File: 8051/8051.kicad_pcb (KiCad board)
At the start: 2 copper layers, 70 x 90 mm, 49 parts, among them J1 GND, J10 C_{OUT}, J2 V_{CC}, J3 OUT TX RX V5 G, J4 S + G, J5 G + CK D, J6 AP-B-C, J7 AN-B-C, J8 A_{OUT}, J9 B_{OUT}, Q1 2N3055, Q2 nfet, Q3 pfet, Q4 2N3055, Q5 nfet, Q6 pfet, Q7 2N3055, Q8 nfet, Q9 pfet, U1 L7805, U2 REGULAR-7133-1, U3 C8051F330

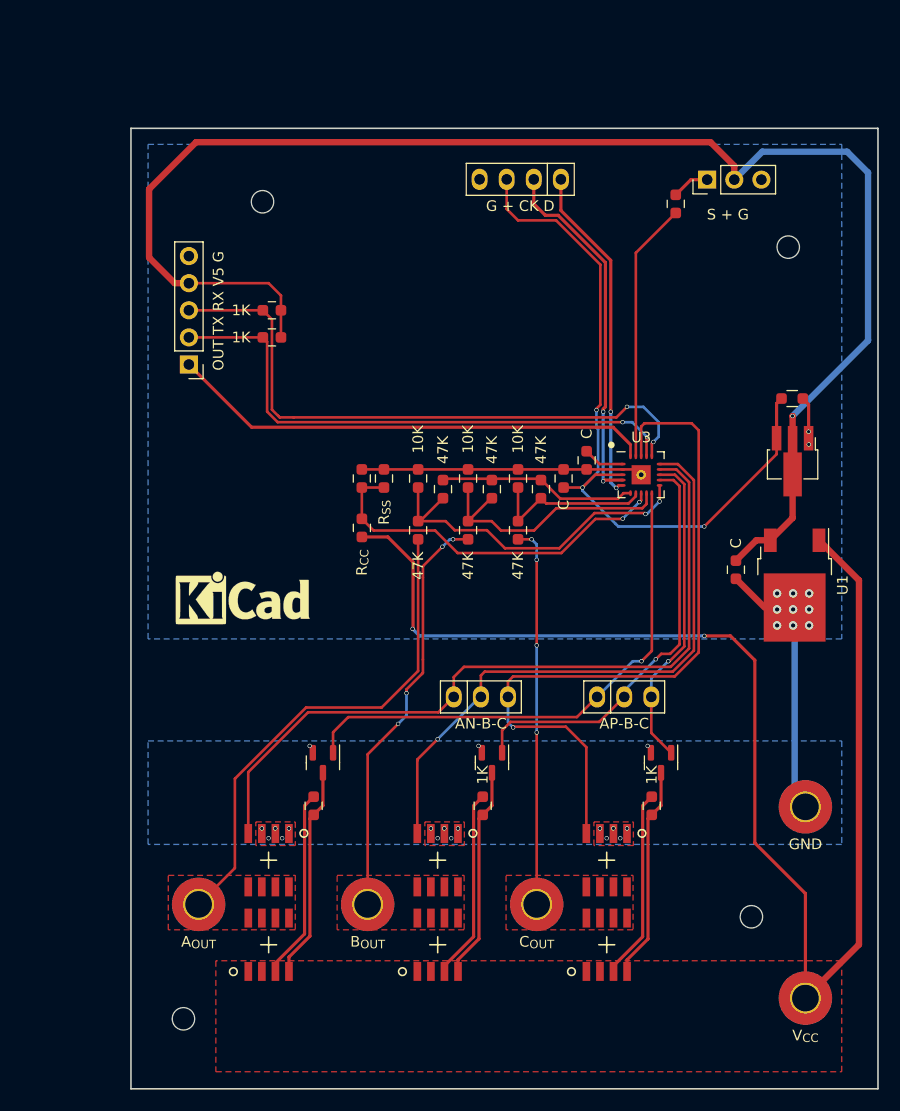
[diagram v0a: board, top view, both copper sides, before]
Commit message: digital module
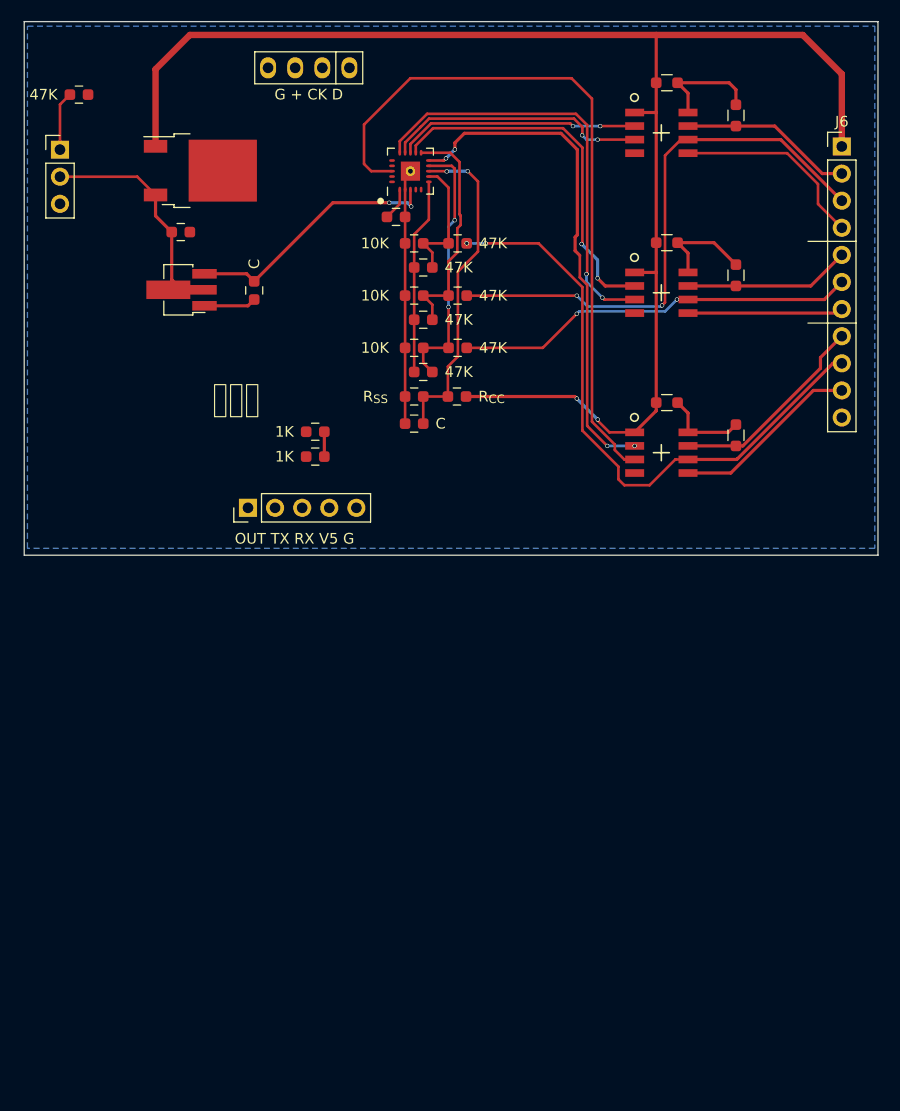
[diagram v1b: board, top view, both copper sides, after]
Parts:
- removed C: 0805_p2.0xpad1.0, footprint:0805_p2.0xpad1.0
- removed J1: GND, MountingHole:MountingHole_2.5mm_Pad_TopBottom
- removed J10: C_{OUT}, MountingHole:MountingHole_2.5mm_Pad_TopBottom
- removed J2: V_{CC}, MountingHole:MountingHole_2.5mm_Pad_TopBottom
- removed J7: AN-B-C, footprint:CONN3-P2.54-DR1.0-W1.5
- removed J8: A_{OUT}, MountingHole:MountingHole_2.5mm_Pad_TopBottom
- removed J9: B_{OUT}, MountingHole:MountingHole_2.5mm_Pad_TopBottom
- removed Q1, Q4, Q7: 2N3055, Package_TO_SOT_SMD:SOT-23
- removed Q2, Q5, Q8: nfet, footprint:SOIC-8
- removed Q3, Q6, Q9: pfet, footprint:SOIC-8
- removed R15, R16, R17: 1K, footprint:0603_p1.7xpad1.0
- removed REF** (x4): MountingHole_2.1mm, MountingHole:MountingHole_2.1mm
- removed REF**: KiCad-Logo_5mm_SilkScreen, Symbol:KiCad-Logo_5mm_SilkScreen
- added C5: C, footprint:0805_p2.0xpad1.0, F.Cu at (86.7, 28.8)
- added C6: C, footprint:0805_p2.0xpad1.0, F.Cu at (86.7, 43.8)
- added C7: C, footprint:0805_p2.0xpad1.0, F.Cu at (86.7, 58.8)
- added D1: D, footprint:0805_p2.0xpad1.0, F.Cu at (80.2, 25.7)
- added D2: D, footprint:0805_p2.0xpad1.0, F.Cu at (80.2, 40.7)
- added D3: D, footprint:0805_p2.0xpad1.0, F.Cu at (80.2, 55.7)
- added U4: IR2103, footprint:SOIC-8, F.Cu at (79.7, 30.4)
- added U5: IR2103, footprint:SOIC-8, F.Cu at (79.7, 45.4)
- added U6: IR2103, footprint:SOIC-8, F.Cu at (79.7, 60.4)
- J3: value OUT TX RX V5 G -> S + G; footprint Connector_PinHeader_2.54mm:PinHeader_1x05_P2.54mm_Vertical -> Connector_PinHeader_2.54mm:PinHeader_1x03_P2.54mm_Vertical
- J4: value S + G -> OUT TX RX V5 G; footprint Connector_PinHeader_2.54mm:PinHeader_1x03_P2.54mm_Vertical -> Connector_PinHeader_2.54mm:PinHeader_1x05_P2.54mm_Vertical
- J6: value AP-B-C -> Conn_01x11; footprint footprint:CONN3-P2.54-DR1.0-W1.5 -> Connector_PinHeader_2.54mm:PinHeader_1x11_P2.54mm_Vertical
- R11: value 47K -> 10K
- R13, R14: value 1K -> 47K
- R3, R4: value 47K -> 1K
- R5: value 10K -> 47K
- moved U1 67.9 mm to (36.5, 34.0), turned to 0 degrees
- moved C2 60.9 mm to (34.7, 39.7), turned to 0 degrees
- moved U2 59.5 mm to (34.7, 45.1), turned to 180 degrees
- moved J6 55.5 mm to (96.6, 31.7)
- moved J4 52.9 mm to (41.0, 65.6)
- moved R5 48.0 mm to (25.1, 26.8), turned to 0 degrees
- moved R14 45.9 mm to (57.4, 47.9), turned to 180 degrees
- moved R13 41.9 mm to (57.4, 52.8), turned to 180 degrees
- moved R3 40.0 mm to (47.3, 58.4), turned to 0 degrees
- moved U3 35.7 mm to (56.2, 34.0), turned to 90 degrees
- moved C3 33.9 mm to (41.5, 45.2), turned to -90 degrees
- moved C1 29.0 mm to (54.8, 38.3), turned to 0 degrees
- moved R10 24.3 mm to (60.6, 40.8), turned to 180 degrees
- moved R11 24.2 mm to (56.5, 40.8), turned to 180 degrees
- moved J3 23.5 mm to (23.4, 32.0), turned to 0 degrees
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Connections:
- J3 pad 1: CPOUT -> Net-(J3-Pad1)
- J3 pad 2: TXD -> +5V
- J3 pad 3: RXD -> GND
- J4 pad 1: Net-(J4-Pad1) -> CPOUT
- J4 pad 2: +5V -> TXD
- J4 pad 3: GND -> RXD
- J6 pad 1: AP -> VCC
- J6 pad 2: BP -> DAP
- J6 pad 3: CP -> AOUT
- R10 pad 1: FC -> COUT
- R10 pad 2: F_ABC -> FC
- R11 pad 1: FB -> FC
- R11 pad 2: F_ABC -> GND
- R12 pad 1: FA -> FC
- R13 pad 1: VCC -> FB
- R13 pad 2: Net-(Q1-Pad3) -> F_ABC
- R14 pad 1: VCC -> FA
- R14 pad 2: Net-(Q4-Pad3) -> F_ABC
- R3 pad 1: Net-(J4-Pad1) -> TXD
- R3 pad 2: RCP -> +5V
- R4 pad 1: AOUT -> RXD
- R4 pad 2: FA -> +5V
- R5 pad 1: FA -> Net-(J3-Pad1)
- R5 pad 2: GND -> RCP
- R6 pad 1: BOUT -> AOUT
- R6 pad 2: FB -> FA
- R7 pad 1: FB -> FA
- R8 pad 1: COUT -> BOUT
- R8 pad 2: FC -> FB
- R9 pad 1: FC -> FB
- U3 pad 10: AP -> CP
- U3 pad 13: CP -> AP
- U3 pad 19: RCP -> CPOUT
- U3 pad 20: CPOUT -> RCP
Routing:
- net +5V: track 139.7 -> 21.9 mm, vias 1 -> 0
- net RXD: track 57.6 -> 0.00 mm, vias 2 -> 0
- net TXD: track 52.5 -> 0.00 mm, vias 2 -> 0
- net AN: track 71.8 -> 24.7 mm, vias 0 -> 2
- net CPOUT: track 45.6 -> 0.00 mm
- net +3V3: track 69.5 -> 24.5 mm, vias 3 -> 2
- net VCC: track 179.1 -> 140.5 mm
- net CK: track 33.7 -> 0.00 mm, vias 2 -> 0
- net 2D: track 31.8 -> 0.00 mm, vias 2 -> 0
- net AP: track 49.7 -> 22.7 mm, vias 1 -> 2
- net GND: track 54.6 -> 28.1 mm, vias 29 -> 0
- net RCP: track 24.4 -> 0.00 mm
- net COUT: track 35.7 -> 57.8 mm, vias 4 -> 2
- net Net-(Q4-Pad3): track 20.4 -> 0.00 mm
- net Net-(Q1-Pad3): track 20.0 -> 0.00 mm
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- removed copper zone on F.Cu, net AOUT
- removed copper zone on F.Cu, net BOUT
- removed copper zone on F.Cu, net COUT
- removed copper zone on F.Cu, net GND
- removed copper zone on F.Cu, net VCC
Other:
- board size 70 x 90 mm -> 80 x 50 mm
- board text added: "保護傘"
